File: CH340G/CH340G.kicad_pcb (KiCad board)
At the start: 2 copper layers, 25.4 x 15.5 mm, 20 parts, among them J1 USB_B_Micro, J2 Conn_01x06

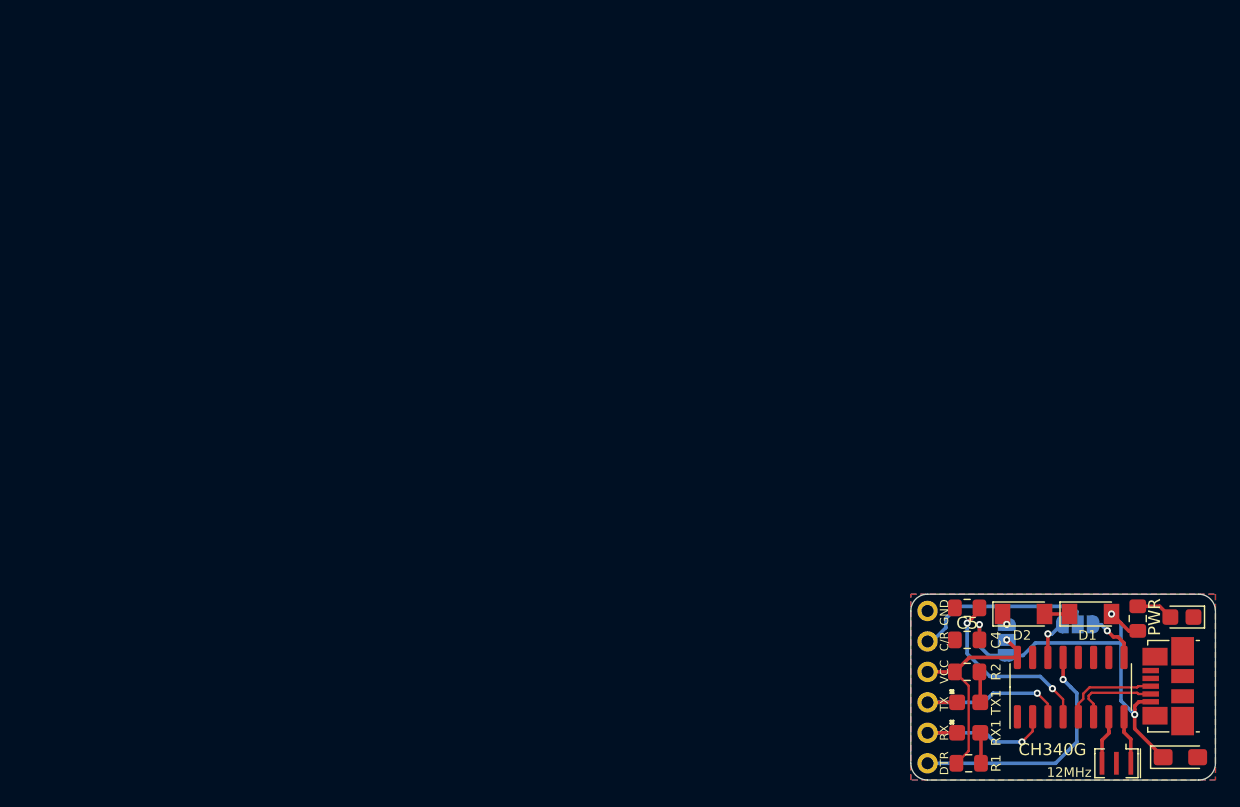
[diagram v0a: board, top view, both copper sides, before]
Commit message: Page Settings Updated
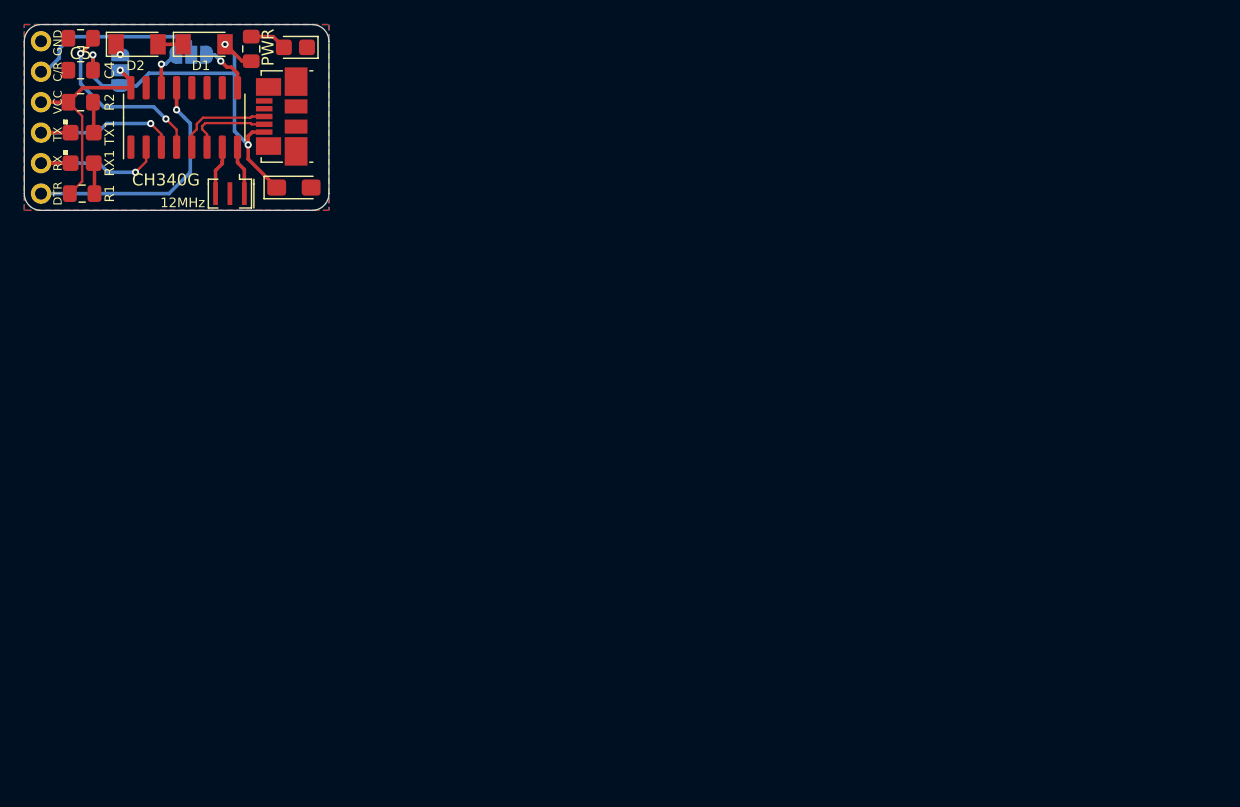
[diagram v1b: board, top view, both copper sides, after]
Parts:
- moved C4 87.9 mm to (61.5, 43.8)
- moved D1 87.9 mm to (71.8, 41.7)
- moved G*** 87.9 mm to (70.6, 51.1)
- moved J2 87.9 mm to (58.2, 54.1)
- moved JP1 87.9 mm to (64.8, 43.8)
- moved JP2 87.9 mm to (70.7, 42.5)
- moved R2 87.9 mm to (61.5, 46.5)
- moved 12MHz 87.9 mm to (73.9, 54.1)
- moved C3 87.9 mm to (79.2, 53.6)
- moved C5 87.9 mm to (61.5, 41.1)
- moved CH340G 87.9 mm to (70.1, 47.8)
- moved D2 87.9 mm to (66.2, 41.7)
- moved G*** 87.9 mm to (63.5, 51.1)
- moved G*** 87.9 mm to (79.5, 47.8)
- moved J1 87.9 mm to (78.2, 47.7)
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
